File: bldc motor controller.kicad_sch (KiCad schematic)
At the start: 53 parts, among them J1 Conn_01x04_Pin, U1 C47023655, U2 ISM330DHCXTR, U3 C529358, U6 LIS2MDLTR

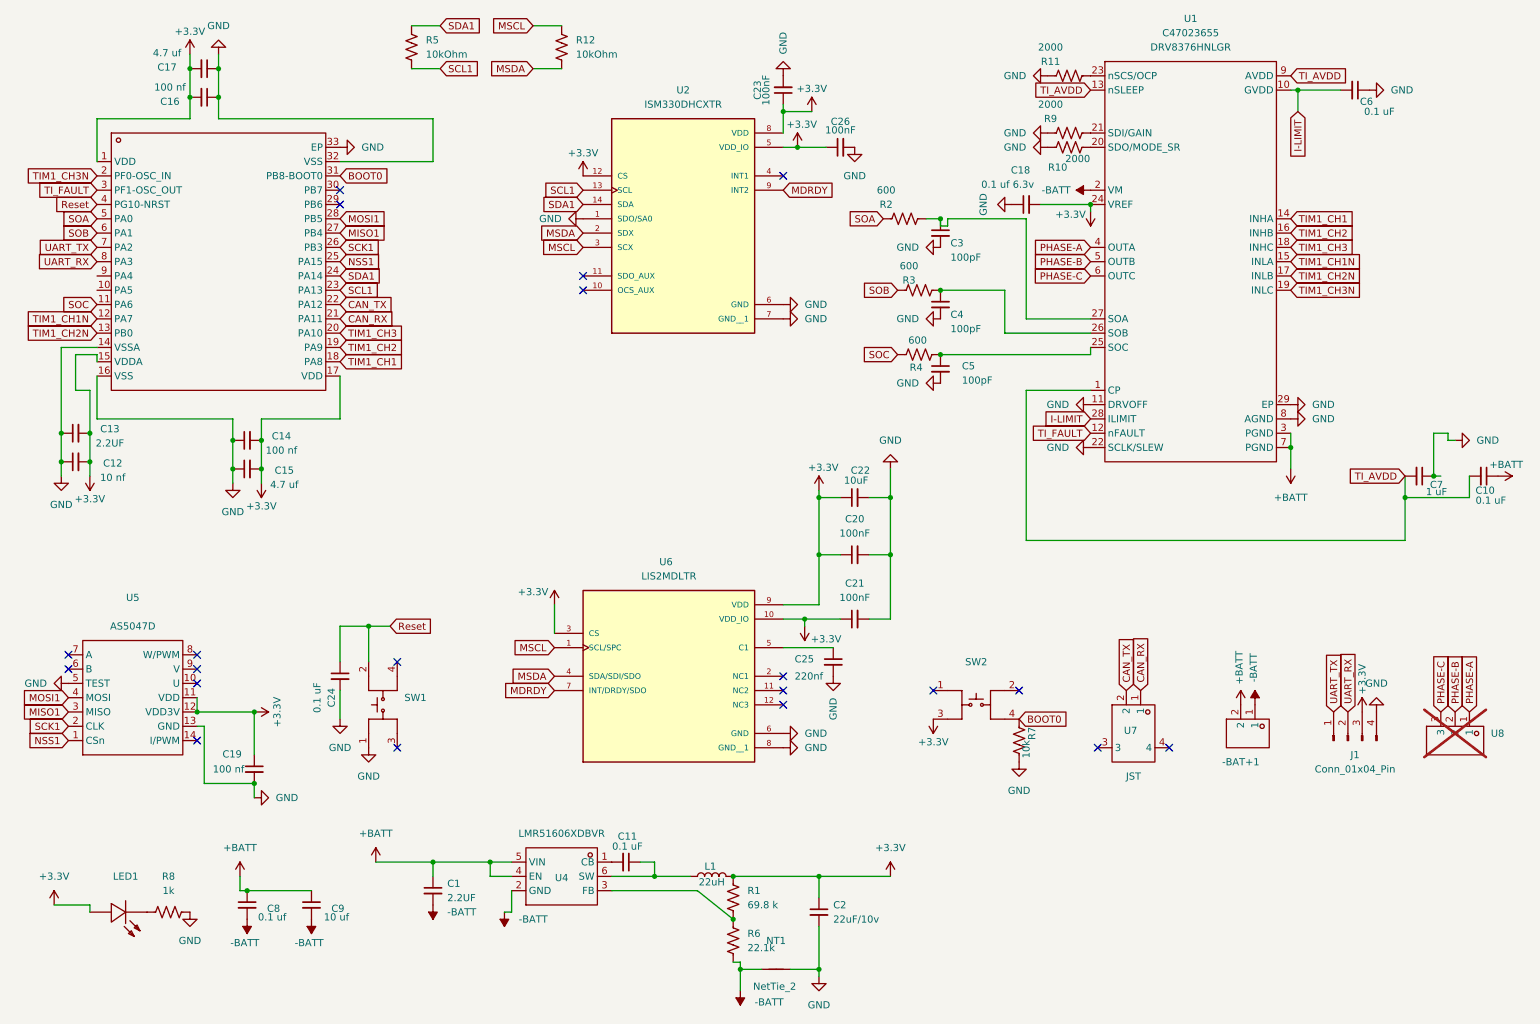
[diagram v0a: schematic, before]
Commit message: Wooo added a can transciever
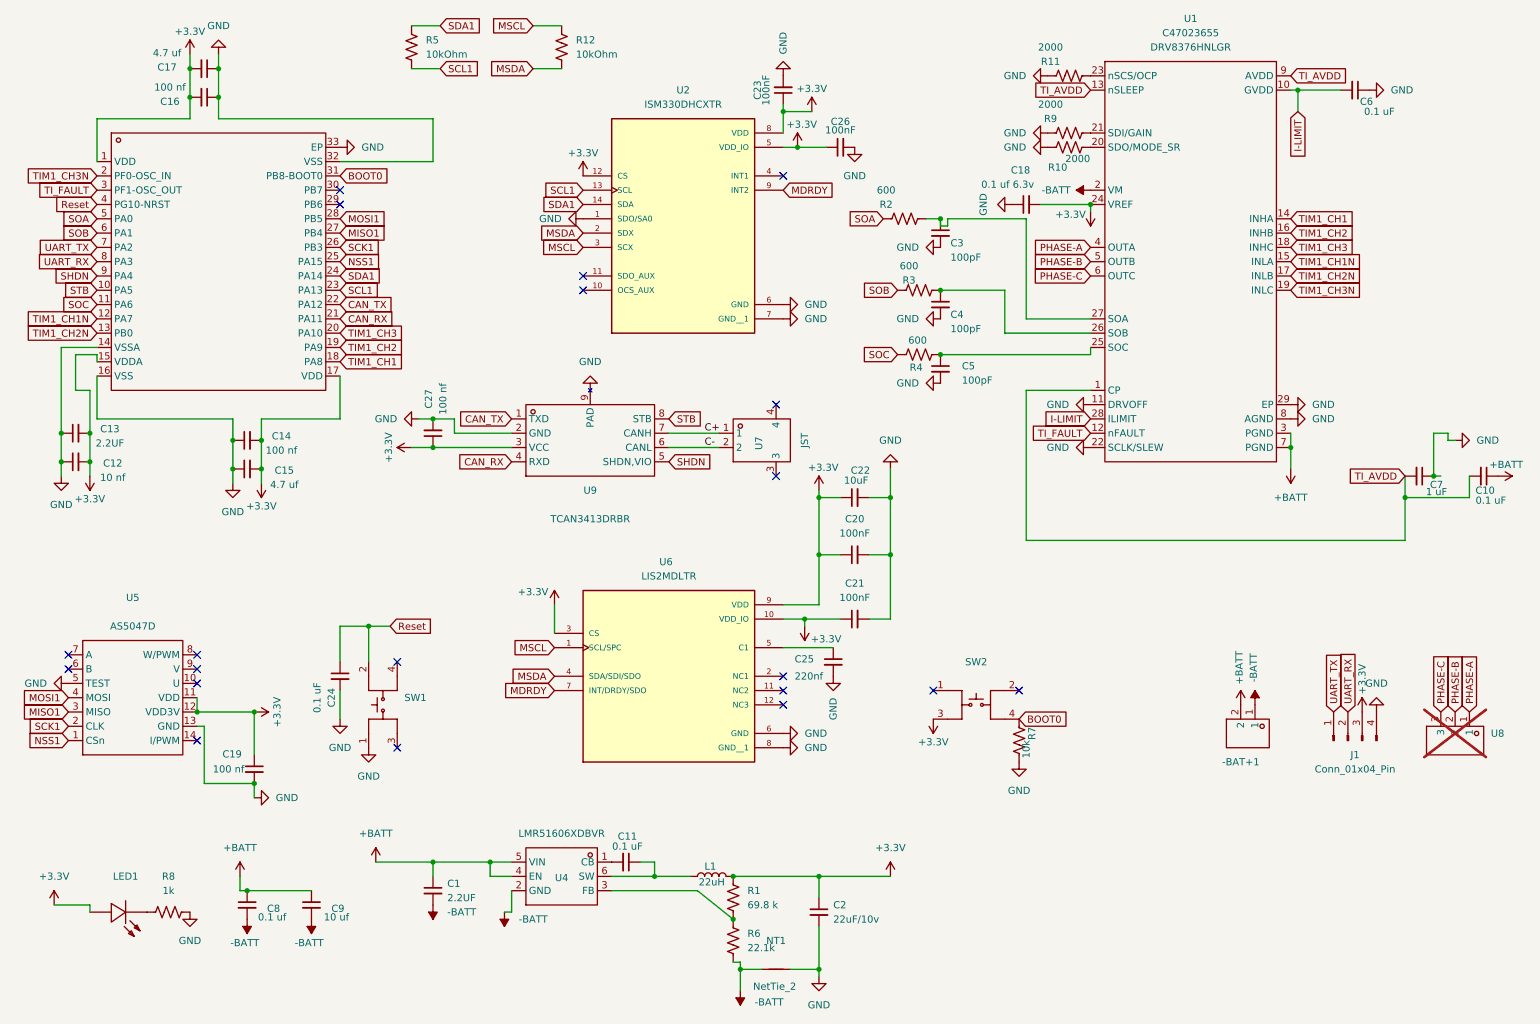
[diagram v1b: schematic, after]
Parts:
- added C27: 100 nf, Capacitor_SMD:C_01005_0402Metric, symbol Device:C_Small
- added U9: ~, bldc-motor-footprints:SON-8_L3.0-W3.0-P0.65-LS2.9-BL-EP, symbol bldc controller:TCAN3413DRBR
- J1: now in the parts list
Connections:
- net +3.3V: now also C27.1, U9.3 (VCC)
- net CAN_RX: now also U9.4 (RXD); no longer U7.1
- net CAN_TX: now also U9.1 (TXD); no longer U7.2
- net GND: now also C27.2, U9.2 (GND), U9.9 (PAD)
- net STB: now reaches U3.10 (PA5)
- net STB: now also U9.8 (STB)
- net SHDN: now reaches U3.9 (PA4)
- net SHDN: now also U9.5 (SHDN,VIO)
- new net C+: U7.1, U9.7 (CANH)
- new net C-: U7.2, U9.6 (CANL)
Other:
- moved on the sheet: U7
